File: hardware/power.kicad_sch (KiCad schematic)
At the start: 55 parts, among them J15 Conn_01x02, Q13 AO3401A, Q14 BC817W, U10 FP6151XR-G1, U7 ZTP7193MA, U8 ZTP7193MA

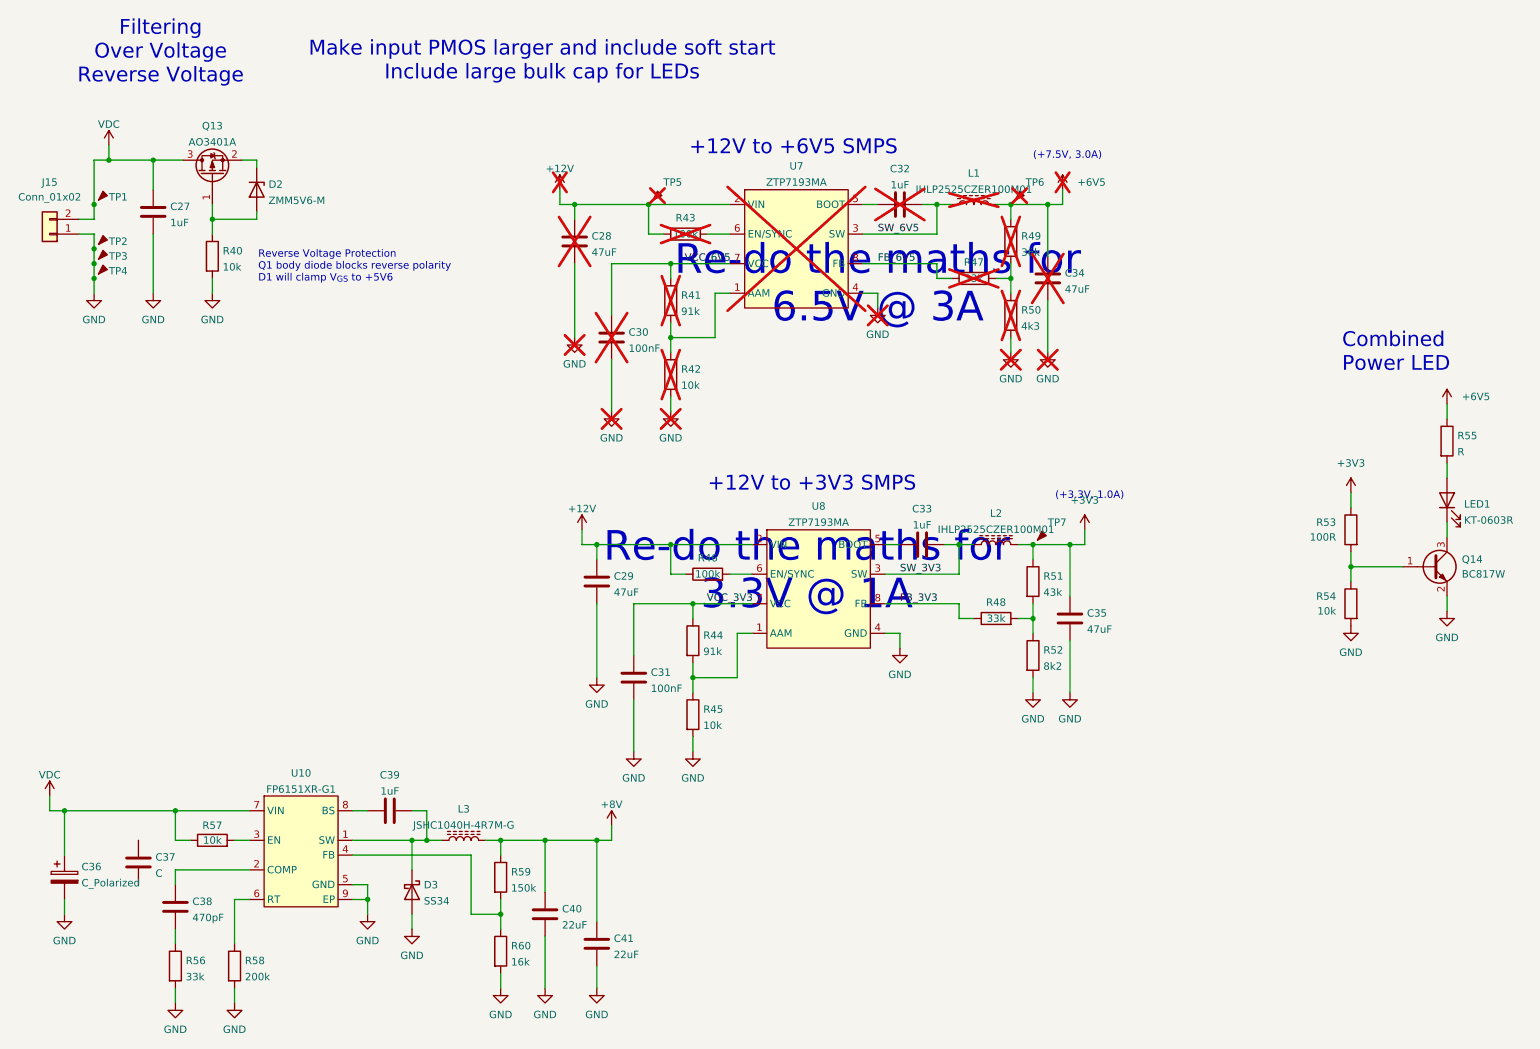
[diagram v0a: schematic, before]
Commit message: fixing issues, adding parts
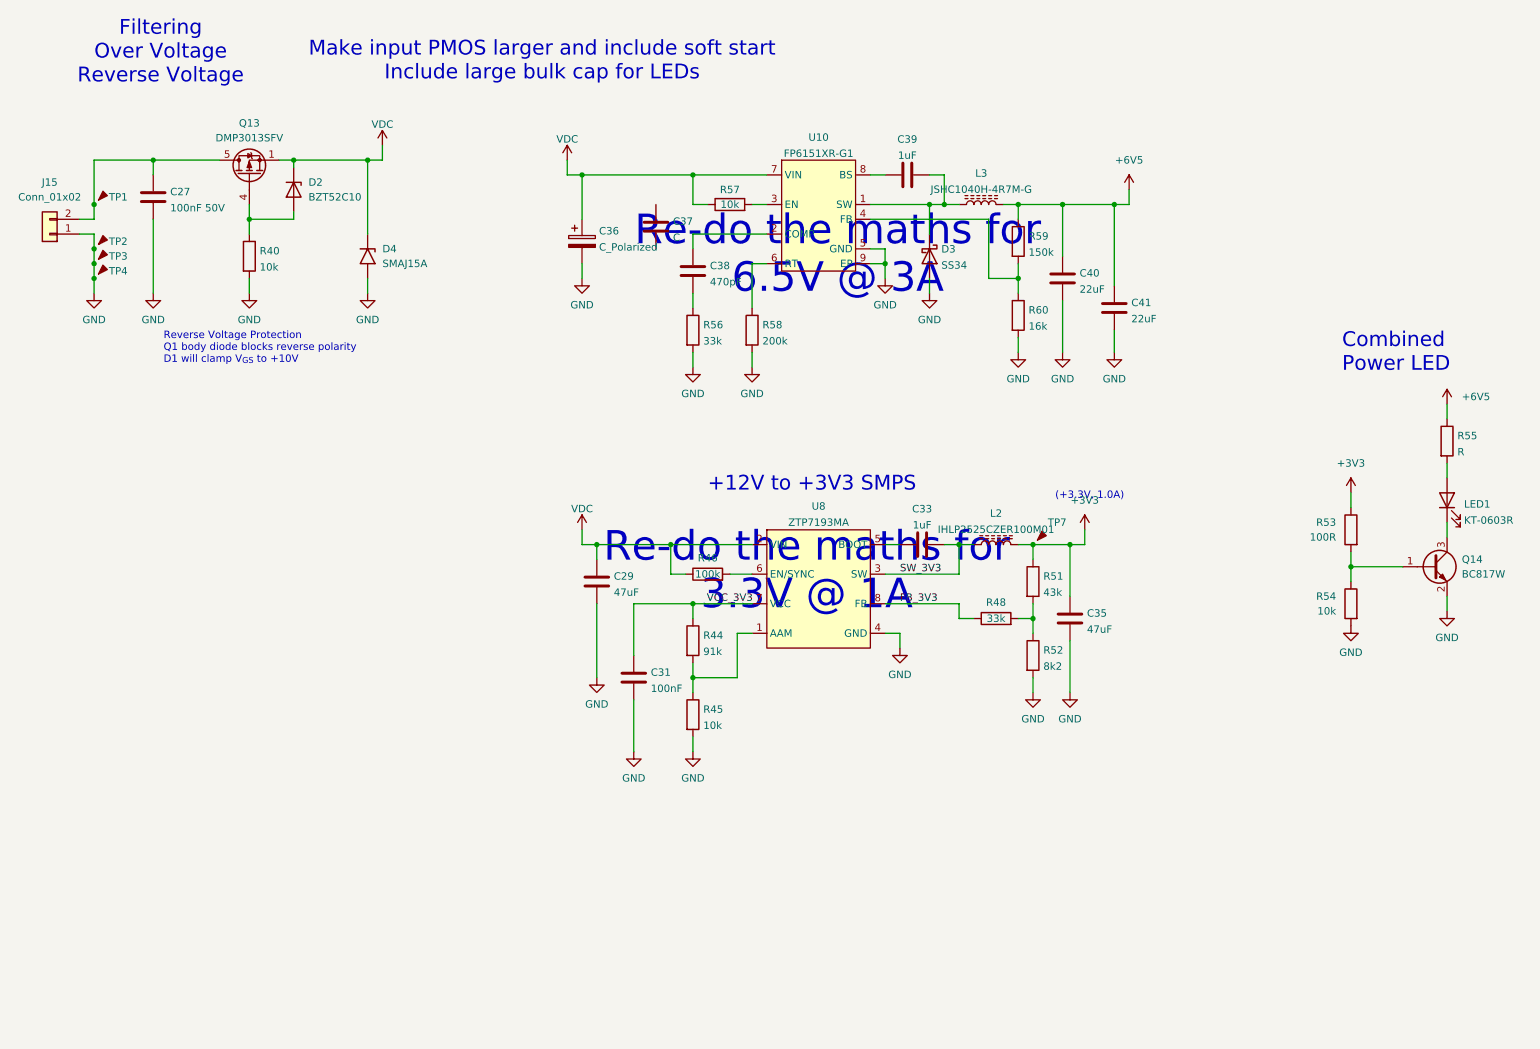
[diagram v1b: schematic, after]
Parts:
- removed C28, C34: 47uF, Capacitor_SMD:C_1210_3225Metric, symbol Device:C
- removed C30: 100nF, Capacitor_SMD:C_0603_1608Metric, symbol Device:C
- removed C32: 1uF, Capacitor_SMD:C_0603_1608Metric, symbol Device:C
- removed L1: IHLP2525CZER100M01, Inductor_SMD:L_Vishay_IHLP-2525, symbol Device:L_Ferrite
- removed Q13: AO3401A, Package_TO_SOT_SMD:SOT-23, symbol Device:Q_PMOS_GSD
- removed R41: 91k, Resistor_SMD:R_0603_1608Metric, symbol Device:R
- removed R42: 10k, Resistor_SMD:R_0603_1608Metric, symbol Device:R
- removed R43: 100k, Resistor_SMD:R_0603_1608Metric, symbol Device:R
- removed R47: 33k, Resistor_SMD:R_0603_1608Metric, symbol Device:R
- removed R49: 36k, Resistor_SMD:R_0603_1608Metric, symbol Device:R
- removed R50: 4k3, Resistor_SMD:R_0603_1608Metric, symbol Device:R
- removed TP5, TP6: TestPoint, TestPoint:TestPoint_Pad_D1.5mm, symbol Pinski1_Parts:TestPoint
- removed U7: ZTP7193MA, Package_TO_SOT_SMD:SOT-23-8, symbol Pinski1_Parts:ZTP7193MA
- added D4: SMAJ15A, Diode_SMD:D_SMA, symbol Diode:SMAJ15A
- added Q13: DMP3013SFV, Package_SON:Diodes_PowerDI3333-8, symbol Transistor_FET:DMP3013SFV
- C27: value 1uF -> 100nF 50V; LCSC C15849 -> (none); Voltage 50V -> (none)
- D2: value ZMM5V6-M -> BZT52C10; footprint Diode_SMD:D_MiniMELF -> Diode_SMD:D_SOD-123; LCSC C8062 -> C19077408
- Q14: LCSC (none) -> C75566
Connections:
- net +12V is gone; now on net VDC: C29.1, R46.1, U8.2 (VIN)
- net +8V is gone; now on net +6V5: C40.1, C41.1, L3.2, R59.1
- net GND: now also D4.2 (A2)
- net VDC: now also D2.1 (K), D4.1 (A1), Q13.1 (S), Q13.2 (S), Q13.3 (S); no longer C27.1, J15.2 (Pin_2), TP1.1
- net at D2.2 (A), R40.1: now also Q13.4 (G)
- new net: C27.1, J15.2 (Pin_2), Q13.5 (D), TP1.1
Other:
- note added: "Reverse Voltage Protection Q1 body diode blocks reverse polarity D1 will clamp V_{GS} to +10V"
- note removed: "(+7.5V, 3.0A)"
- note removed: "+12V to +6V5 SMPS"
- note removed: "Reverse Voltage Protection Q1 body diode blocks reverse polarity D1 will clamp V_{GS} to +5V6"
- moved on the sheet: C27, C36, C37, C38, C39, C40, C41, D3, L3, R40, R56, R57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
